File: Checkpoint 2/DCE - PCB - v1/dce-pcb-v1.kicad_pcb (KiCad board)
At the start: 2 copper layers, 83.3 x 51.5 mm, 56 parts, among them J1 Conn_01x06_Socket, J2 Conn_01x02_Socket, J3 Conn_01x02_Socket, M1 2N7000, Q1 BC547B, Q2 BC547B, Q3 BC547B, Q4 BC557B, Q5 BC557B, Q6 BC547B, Q7 TIP41C, Q8 TIP42C, Q9 BC547B, U1 LM324

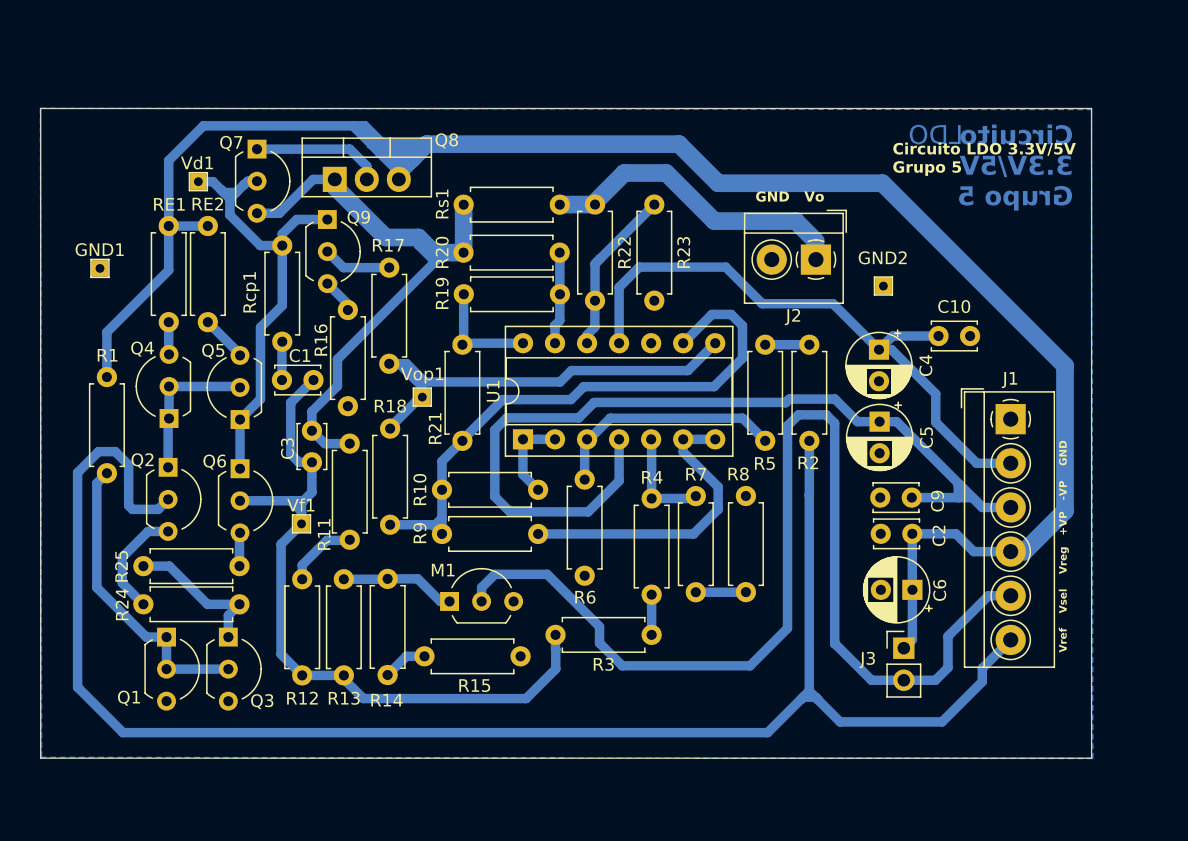
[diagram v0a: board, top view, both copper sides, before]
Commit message: ojala no rompa todo
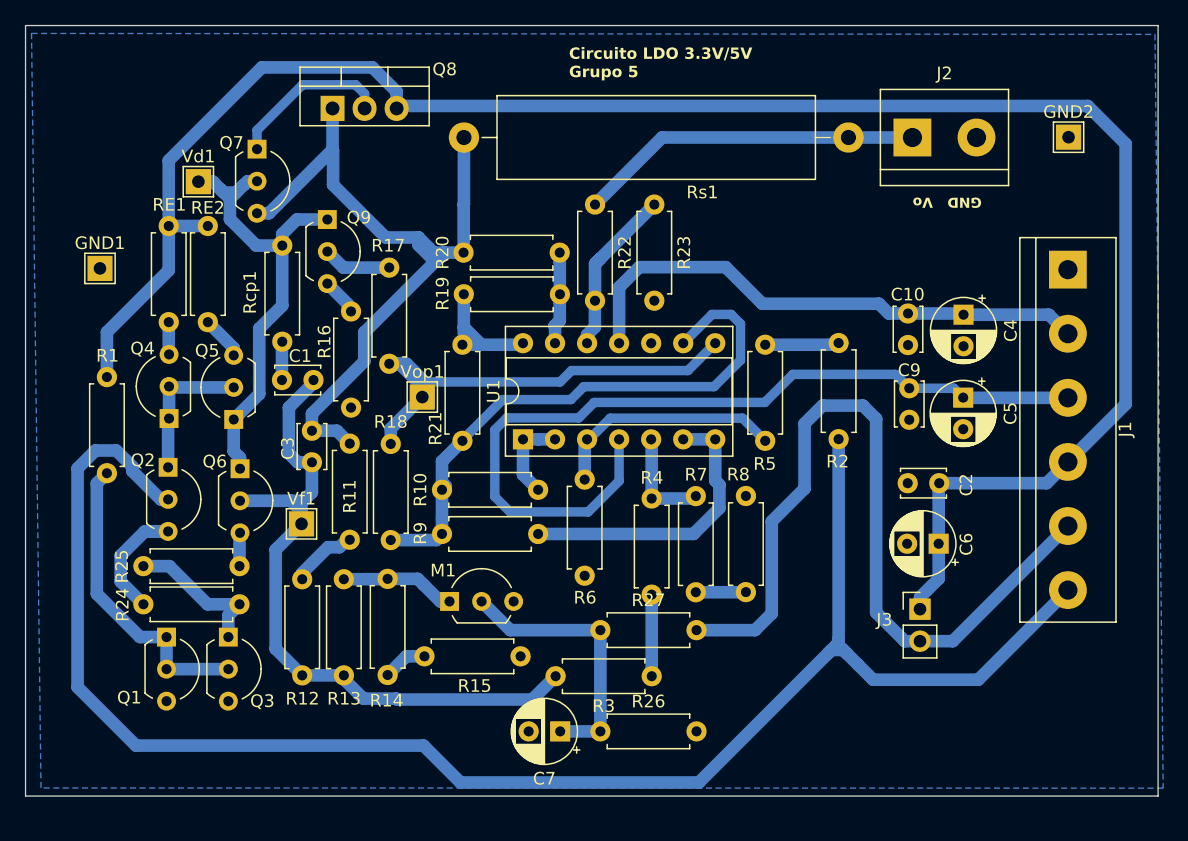
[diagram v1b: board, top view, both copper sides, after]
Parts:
- added C7: C, Capacitor_THT:CP_Radial_D5.0mm_P2.50mm, F.Cu at (160.6, 94.4)
- added R26: 1k, Resistor_THT:R_Axial_DIN0207_L6.3mm_D2.5mm_P7.62mm_Horizontal, F.Cu at (163.8, 94.4)
- added R27: 1k, Resistor_THT:R_Axial_DIN0207_L6.3mm_D2.5mm_P7.62mm_Horizontal, F.Cu at (163.8, 86.4)
- GND1, GND2, Vd1, Vf1, Vop1: footprint LDO_C2:TestPoint_THTPad_1.3x1.3mm_Drill0.7mm -> TestPoint:TestPoint_THTPad_2.0x2.0mm_Drill1.0mm
- J1: footprint LDO_C2:TerminalBlock_4Ucon_1x06_P3.50mm_Horizontal -> TerminalBlock:TerminalBlock_bornier-6_P5.08mm
- J2: footprint LDO_C2:TerminalBlock_4Ucon_1x02_P3.50mm_Horizontal(3D) -> TerminalBlock:TerminalBlock_bornier-2_P5.08mm
- Rs1: footprint Resistor_THT:R_Axial_DIN0207_L6.3mm_D2.5mm_P7.62mm_Horizontal -> Resistor_THT:R_Axial_Power_L25.0mm_W6.4mm_P30.48mm
- moved Rs1 23.5 mm to (183.4, 47.3)
- moved GND2 18.8 mm to (200.9, 47.3)
- moved J1 12.7 mm to (200.8, 57.8)
- moved J2 12.3 mm to (188.5, 47.3), turned to 0 degrees
- moved C9 8.67 mm to (188.2, 67.2), turned to -90 degrees
- moved C4 7.25 mm to (192.6, 61.4)
- moved C5 6.89 mm to (192.5, 67.9)
- moved Q8 5.63 mm to (142.5, 45.0)
- moved C2 4.55 mm to (190.6, 74.7)
- moved C6 4.21 mm to (190.6, 79.5)
- moved J3 3.35 mm to (189.1, 84.7)
- moved R3 3.28 mm to (167.8, 90.0)
- moved C10 3.01 mm to (188.2, 61.3), turned to -90 degrees
- moved R2 2.32 mm to (182.7, 63.6)
- moved R18 1.22 mm to (147.2, 79.2)
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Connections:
- M1 pad 2: /Vsel -> Net-(M1-G)
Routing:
- net /Vsel: track 87.5 -> 64.6 mm
- net Net-(M1-G): track 0.00 -> 21.6 mm
- net Net-(Q7-E): track 48.8 -> 60.2 mm
- net /-VPOSA: track 49.1 -> 42.9 mm
- net /+VPOSA: track 72.5 -> 68.0 mm
- net /Vref: track 131.5 -> 135.2 mm
- net Net-(R3-Pad1): track 3.19 -> 6.50 mm
- net Net-(R19-Pad2): track 8.19 -> 11.0 mm
- net Net-(Q7-C): track 10.3 -> 13.0 mm
- net Net-(R2-Pad1): track 3.50 -> 6.03 mm
- net /Vo: track 25.1 -> 27.5 mm
- net /Vf: track 58.1 -> 55.7 mm
- net /Sum: track 47.4 -> 46.2 mm
- net Net-(R17-Pad1): track 35.8 -> 36.9 mm
- net Net-(Q2-E): track 8.90 -> 9.97 mm
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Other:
- board size 83.3 x 51.5 mm -> 89.8 x 61.1 mm
- board text removed: "Circuito 3.3V/5V Grupo 5"
- board text removed: "LDO"
- board text removed: "Vref Vsel Vreg +VP -VP GND"

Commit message: nuevo pcb
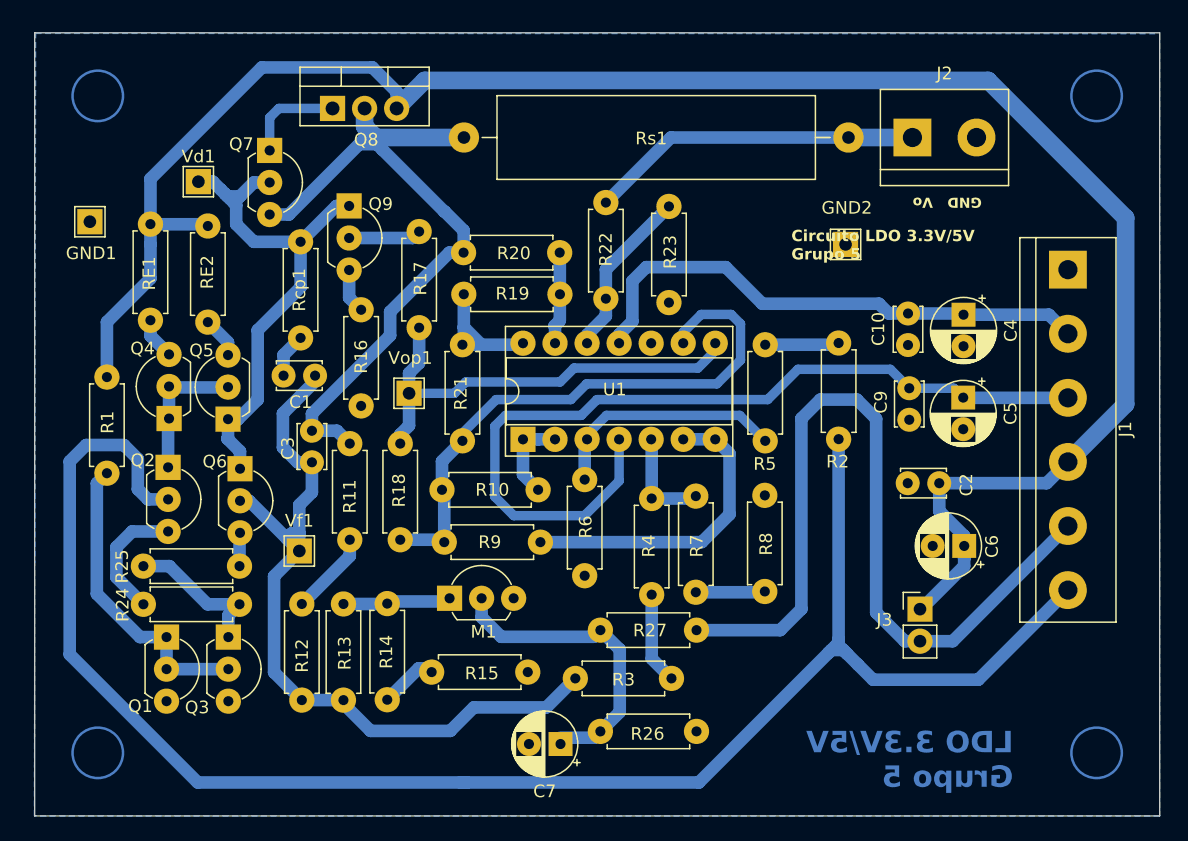
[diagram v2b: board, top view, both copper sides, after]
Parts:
- moved GND2 19.6 mm to (183.2, 55.8)
- moved GND1 3.79 mm to (123.3, 54.0)
- moved R17 3.71 mm to (149.4, 62.4)
- moved Vf1 2.16 mm to (139.9, 80.1)
- moved Q9 2.03 mm to (143.8, 52.8)
- moved C6 2.03 mm to (192.6, 79.7)
- moved R13 1.96 mm to (143.4, 91.9)
- moved R12 1.96 mm to (140.1, 84.3)
- moved R14 1.96 mm to (146.9, 84.3)
- moved R3 1.57 mm to (169.4, 90.2)
- moved R8 1.50 mm to (176.8, 83.3)
- moved Rcp1 1.48 mm to (140.0, 55.6)
- moved RE1 1.46 mm to (128.1, 54.2)
- moved R15 1.37 mm to (150.4, 89.7)
- moved R23 1.17 mm to (169.2, 52.8)
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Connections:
- Q8 pad 1: Net-(Q7-E) -> Net-(Q7-C)
- Q8 pad 2: Net-(Q7-C) -> Net-(Q7-E)
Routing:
- net /Vf: track 55.7 -> 62.9 mm
- net Net-(Q7-C): track 13.0 -> 7.89 mm
- net /Vlc: track 38.2 -> 41.6 mm
- net Net-(M1-G): track 21.6 -> 24.2 mm
- net /Vref: track 135.2 -> 137.3 mm
- net /Vsel: track 64.6 -> 66.6 mm
- net Net-(R7-Pad2): track 3.97 -> 5.92 mm
- net Net-(R11-Pad2): track 5.36 -> 6.89 mm
- net /Vreg: track 153.3 -> 154.8 mm
- net Net-(U1B--): track 23.3 -> 24.4 mm
- net Net-(R14-Pad2): track 3.53 -> 4.45 mm
- net /Vo: track 27.5 -> 26.7 mm
- net Net-(R17-Pad1): track 36.9 -> 36.1 mm
- net Net-(R3-Pad1): track 6.50 -> 7.32 mm
- net Net-(Q9-E): track 2.77 -> 3.54 mm
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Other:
- board size 89.8 x 61.1 mm -> 89.2 x 62.1 mm
- board text added: "LDO 3.3V/5V Grupo 5"
